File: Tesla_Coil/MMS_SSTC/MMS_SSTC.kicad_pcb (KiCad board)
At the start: 2 copper layers, 100 x 79 mm, 40 parts, among them J1 Screw_Terminal_01x02, J2 Screw_Terminal_01x02, Q1 FQA8N100C, SW2 70C, U1 NE555P, U2 UCC37322P, U3 CD74HC14E, U4 LM7812_TO220, U5 LM7805_TO220

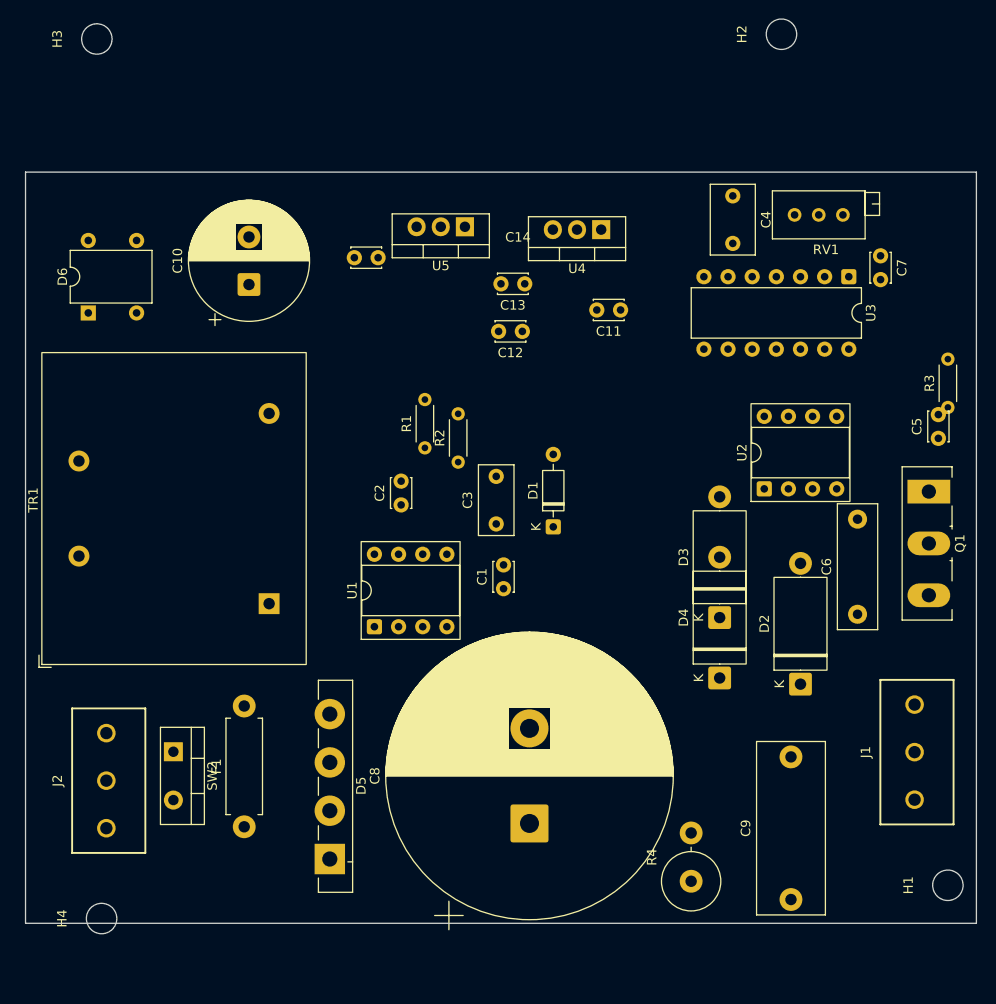
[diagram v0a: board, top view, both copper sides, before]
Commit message: Rough layout on final SSTC PCB
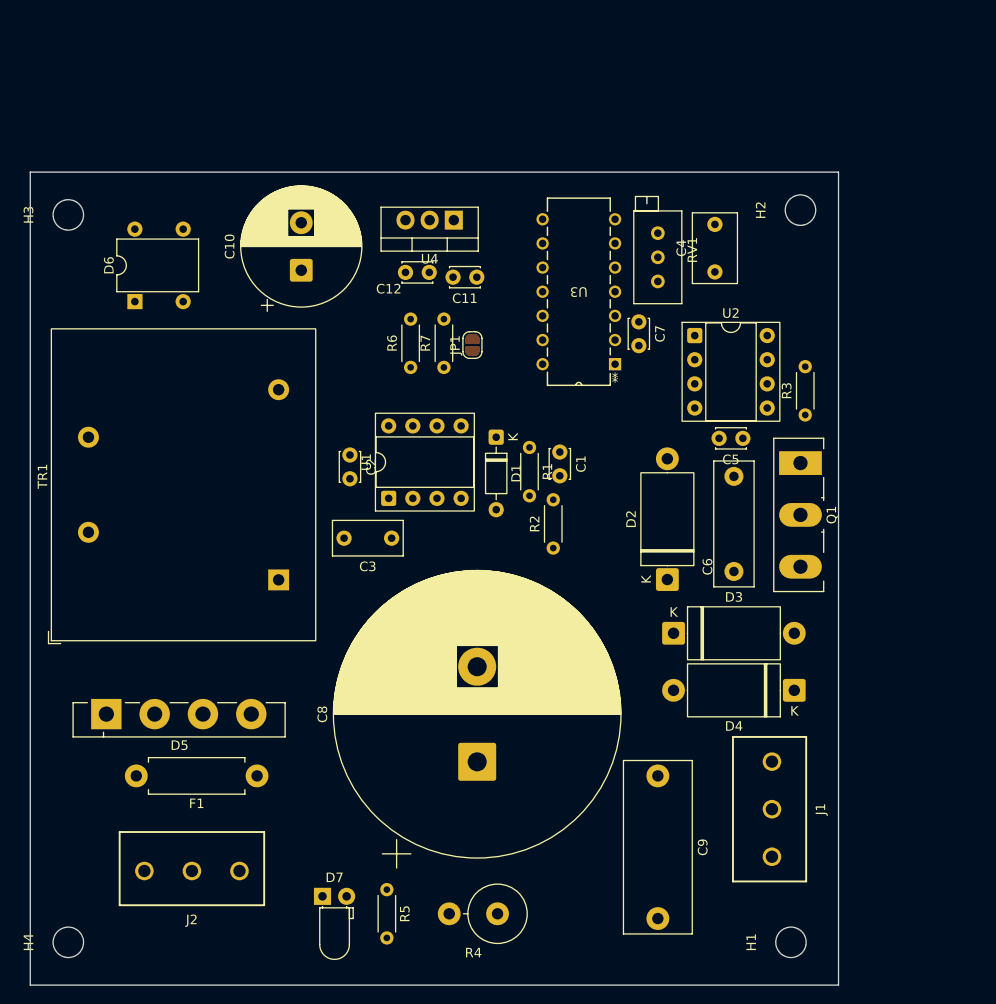
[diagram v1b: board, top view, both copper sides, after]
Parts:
- removed C13, C14: 0.1u, Capacitor_THT:C_Disc_D3.0mm_W2.0mm_P2.50mm
- removed SW2: 70C, Package_TO_SOT_THT:TO-220-2_Vertical
- removed U5: LM7805_TO220, Package_TO_SOT_THT:TO-220-3_Vertical
- added D7: LED, LED_THT:LED_D3.0mm_Horizontal_O1.27mm_Z2.0mm, F.Cu at (90.7, 105.2)
- added JP1: SolderJumper_2_Open, Jumper:SolderJumper-2_P1.3mm_Open_RoundedPad1.0x1.5mm, F.Cu at (106.5, 47.2)
- added R5: 1.2k, Resistor_THT:R_Axial_DIN0204_L3.6mm_D1.6mm_P5.08mm_Horizontal, F.Cu at (97.5, 104.5)
- added R6: 1.8k, Resistor_THT:R_Axial_DIN0204_L3.6mm_D1.6mm_P5.08mm_Horizontal, F.Cu at (100.0, 49.5)
- added R7: 1.5k, Resistor_THT:R_Axial_DIN0204_L3.6mm_D1.6mm_P5.08mm_Horizontal, F.Cu at (103.5, 49.5)
- C8: value 1500u -> 570u
- R4: value 18k -> 8.2k
- RV1: value 10k -> 2.2k
- U3: footprint Package_DIP:DIP-14_W7.62mm -> locals:N14
- moved U3 32.8 mm to (113.9, 34.0), turned to 180 degrees
- moved D5 28.0 mm to (68.0, 86.0), turned to 0 degrees
- moved C7 26.4 mm to (124.0, 44.8)
- moved R4 20.6 mm to (109.1, 107.0), turned to 180 degrees
- moved C5 20.6 mm to (134.9, 57.0), turned to 180 degrees
- moved C9 19.1 mm to (126.0, 92.5), turned to -90 degrees
- moved H3 18.7 mm to (64.0, 33.5)
- moved H2 18.6 mm to (141.0, 33.0)
- moved D2 17.8 mm to (127.0, 71.8)
- moved U2 17.7 mm to (129.9, 46.2), turned to 0 degrees
- moved H1 17.6 mm to (140.0, 110.0)
- moved J1 16.2 mm to (138.0, 96.0), turned to -90 degrees
- moved RV1 16.0 mm to (126.0, 40.5), turned to -90 degrees
- moved C1 15.5 mm to (115.7, 58.4), turned to -90 degrees
- moved U4 15.5 mm to (104.5, 34.0)
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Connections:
- net +5V renamed Net-(JP1-A)
- F1 pad 2: Net-(SW2-A) -> AC_PROT
- R4 pad 2: GND -> Net-(D7-A)
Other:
- board size 100 x 79 mm -> 85 x 85.5 mm

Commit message: Commit progress on final SSTC board
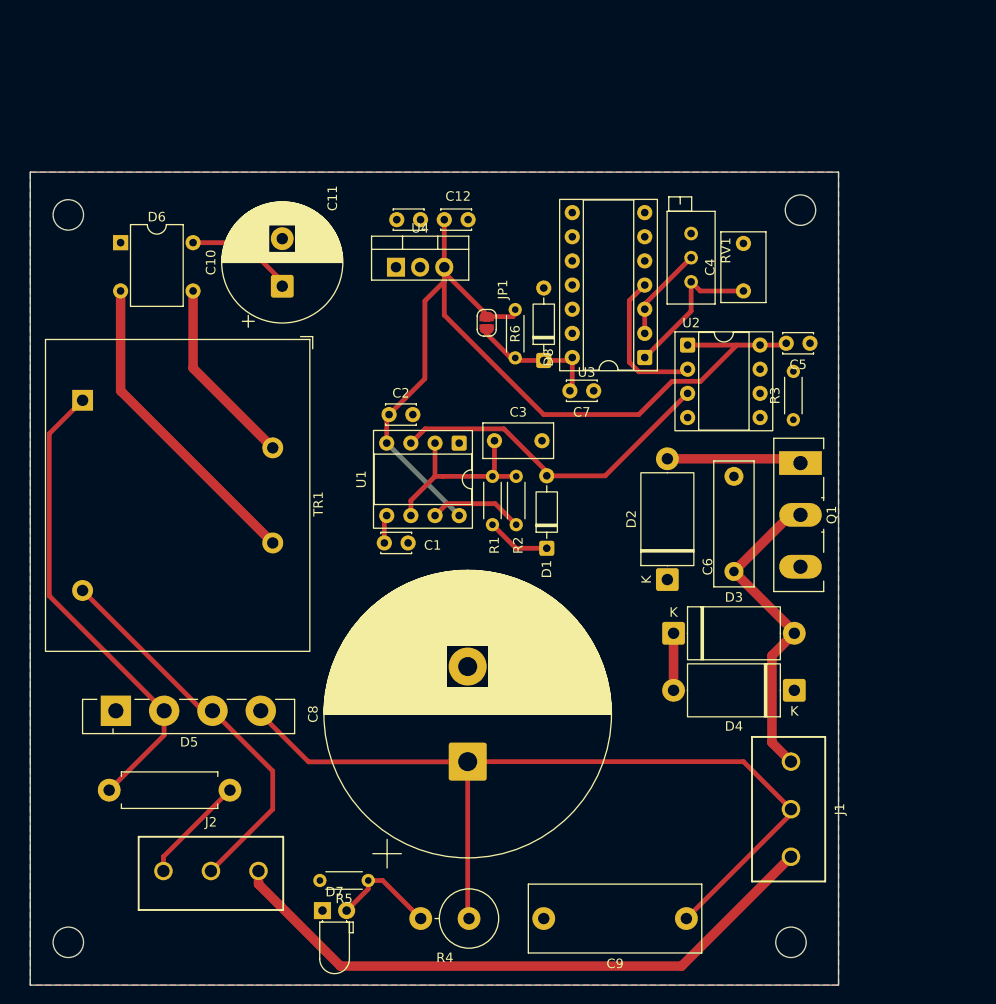
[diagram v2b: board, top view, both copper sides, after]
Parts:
- removed R7: 1.5k, Resistor_THT:R_Axial_DIN0204_L3.6mm_D1.6mm_P5.08mm_Horizontal
- added D8: 5.6V, Diode_THT:D_DO-35_SOD27_P7.62mm_Horizontal, F.Cu at (114.0, 48.8)
- R6: value 1.8k -> 1k
- U3: footprint locals:N14 -> Package_DIP:DIP-14_W7.62mm_Socket
- moved TR1 27.1 mm to (85.5, 53.0), turned to -90 degrees
- moved C1 20.8 mm to (97.2, 68.0), turned to 0 degrees
- moved U3 18.1 mm to (124.6, 48.5)
- moved C9 15.3 mm to (129.0, 107.5), turned to 180 degrees
- moved C3 14.9 mm to (108.8, 57.2), turned to 0 degrees
- moved D1 12.8 mm to (114.3, 68.6), turned to 90 degrees
- moved R6 12.6 mm to (111.0, 43.5), turned to -90 degrees
- moved C5 12.2 mm to (142.0, 47.0)
- moved C11 10.4 mm to (98.5, 34.0), turned to 0 degrees
- moved U1 9.42 mm to (105.1, 57.5), turned to -90 degrees
- moved R1 9.01 mm to (108.6, 66.1), turned to 90 degrees
- moved C7 8.67 mm to (119.2, 52.0), turned to 180 degrees
- moved U4 7.84 mm to (98.5, 39.0), turned to 0 degrees
- moved D6 6.38 mm to (69.5, 36.4), turned to 0 degrees
- moved C2 5.91 mm to (97.7, 54.5), turned to 0 degrees
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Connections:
- net Net-(D2-A2) renamed /GATE
- C6 pad 1: Net-(D3-A2) -> /DRAIN
- D3 pad 2: Net-(D3-A2) -> /DRAIN
- J1 pad 1: Earth -> /DRAIN
- J1 pad 3: Net-(D3-A2) -> Earth
- Q1 pad 2: Net-(D3-A2) -> /DRAIN
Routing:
- net +12V: track 0.00 -> 102.1 mm
- net +170V: track 0.00 -> 93.5 mm
- net Earth: track 0.00 -> 65.7 mm
- net AC_PROT: track 0.00 -> 49.8 mm
- net NEUT: track 0.00 -> 41.1 mm
- net INTERRUPT_OUT: track 0.00 -> 35.7 mm
- net /DRAIN: track 0.00 -> 33.9 mm
- net Net-(D6-Pad2): track 0.00 -> 33.1 mm
- net Net-(U1-THR): track 0.00 -> 21.2 mm
- net Net-(D6-Pad3): track 0.00 -> 20.0 mm
- net Net-(U3-1A): track 0.00 -> 15.9 mm
- net OSC_OUT: track 0.00 -> 15.4 mm
- net Net-(D8-K): track 0.00 -> 14.7 mm
- net /GATE: track 0.00 -> 14.2 mm
- net HT_SW: track 0.00 -> 11.4 mm
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- added copper zone on B.Cu, net GND
- added copper zone on F.Cu, net GND

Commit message: route SSTC PCB and then find out critical problem yay
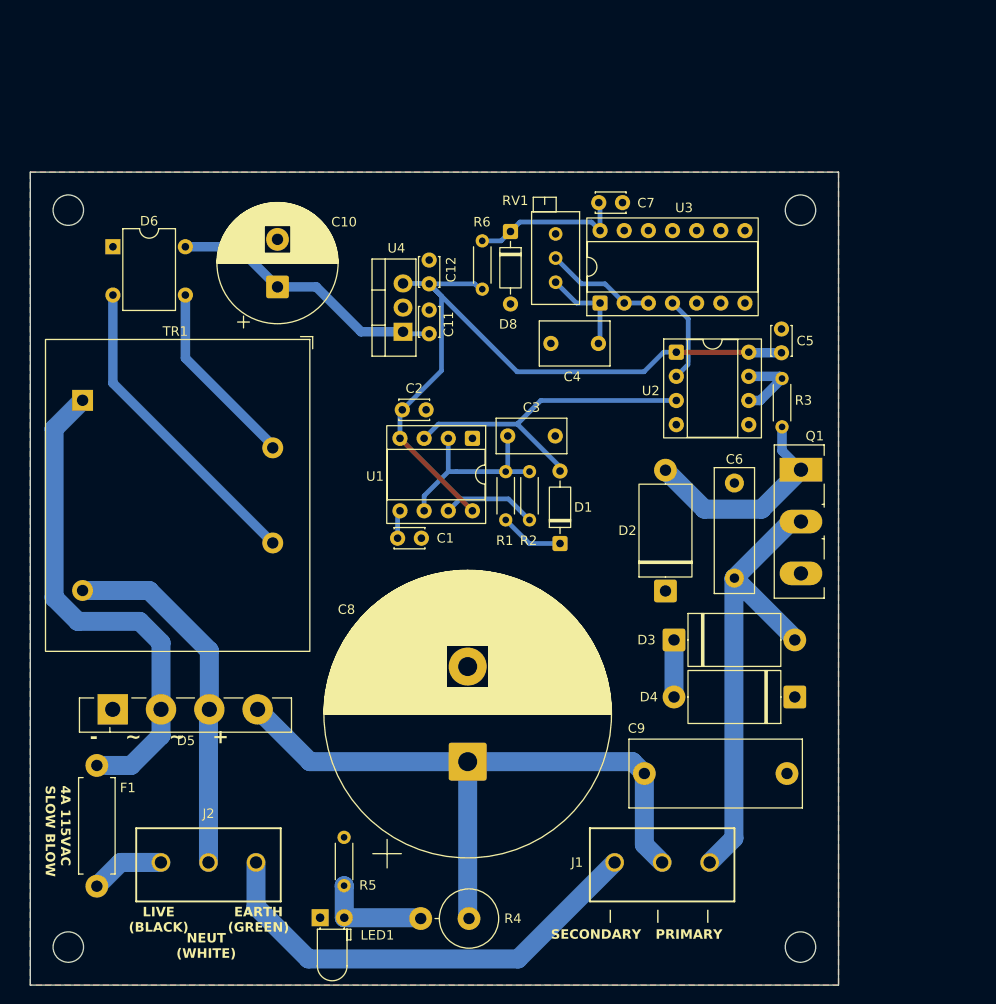
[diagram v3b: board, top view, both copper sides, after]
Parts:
- removed JP1: SolderJumper_2_Open, Jumper:SolderJumper-2_P1.3mm_Open_RoundedPad1.0x1.5mm
- F1: value 4A -> 4A 115VAC SLOW BLOW
- moved C7 20.0 mm to (122.3, 32.2)
- moved F1 17.3 mm to (67.0, 104.1), turned to 90 degrees
- moved C4 16.2 mm to (119.8, 47.0), turned to 180 degrees
- moved C9 15.9 mm to (124.6, 92.2), turned to 0 degrees
- moved J1 14.7 mm to (126.5, 101.6), turned to 0 degrees
- moved RV1 14.3 mm to (115.2, 40.6)
- moved D8 14.0 mm to (110.5, 35.2), turned to -90 degrees
- moved C11 12.5 mm to (102.0, 46.0), turned to 90 degrees
- moved U3 7.41 mm to (119.9, 42.8), turned to 90 degrees
- moved C12 6.93 mm to (102.0, 40.8), turned to 90 degrees
- moved U4 6.83 mm to (99.2, 45.8), turned to 90 degrees
- moved R6 4.08 mm to (107.5, 41.3), turned to 90 degrees
- moved C5 3.35 mm to (139.0, 45.5), turned to -90 degrees
- moved R5 2.60 mm to (93.0, 104.0), turned to 90 degrees
- moved C1 1.48 mm to (98.6, 67.5)
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- renumbered D7 to LED1
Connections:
- J1 pad 1: /DRAIN -> Earth
- J1 pad 3: Earth -> /DRAIN
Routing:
- net +170V: track 93.5 -> 70.1 mm
- net +12V: track 102.1 -> 80.3 mm
- net Net-(D6-+): track 11.4 -> 29.4 mm
- net Earth: track 65.7 -> 48.8 mm
- net /DRAIN: track 33.9 -> 49.6 mm
- net /GATE: track 14.2 -> 23.0 mm
- net Net-(U2-OUT): track 0.00 -> 8.05 mm
- net OSC_OUT: track 15.4 -> 9.06 mm
- net Net-(U3-1A): track 15.9 -> 9.90 mm
- net HT_SW: track 11.4 -> 7.78 mm
- net AC_PROT: track 49.8 -> 53.0 mm
- net NEUT: track 41.1 -> 38.3 mm
- net Net-(D8-K): track 14.7 -> 16.6 mm
- net Net-(U3-1Y): track 9.98 -> 11.7 mm
- net INTERRUPT_OUT: track 35.7 -> 35.0 mm
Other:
- board text added: "- ~ ~ +"
- board text added: "4A 115VAC SLOW BLOW"
- board text added: "EARTH (GREEN)"
- board text added: "LIVE (BLACK)"
- board text added: "NEUT (WHITE)"
- board text added: "PRIMARY"
- board text added: "SECONDARY"
- board text added: "|"
